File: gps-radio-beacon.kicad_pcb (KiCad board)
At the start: 2 copper layers, 106.4 x 69.7 mm, 40 parts, among them J1 Conn_01x16, J2 Conn_01x16, J3 Conn_Coaxial, J4 Conn_Coaxial, J5 Screw_Terminal_01x04, P1 USB_C_Plug_USB2.0, Q1 Q_PMOS_DGS, U1 PGA2040, U2 RFM95W-915S2, U3 MAX-M10S, U4 NCP1117-3.3_SOT223

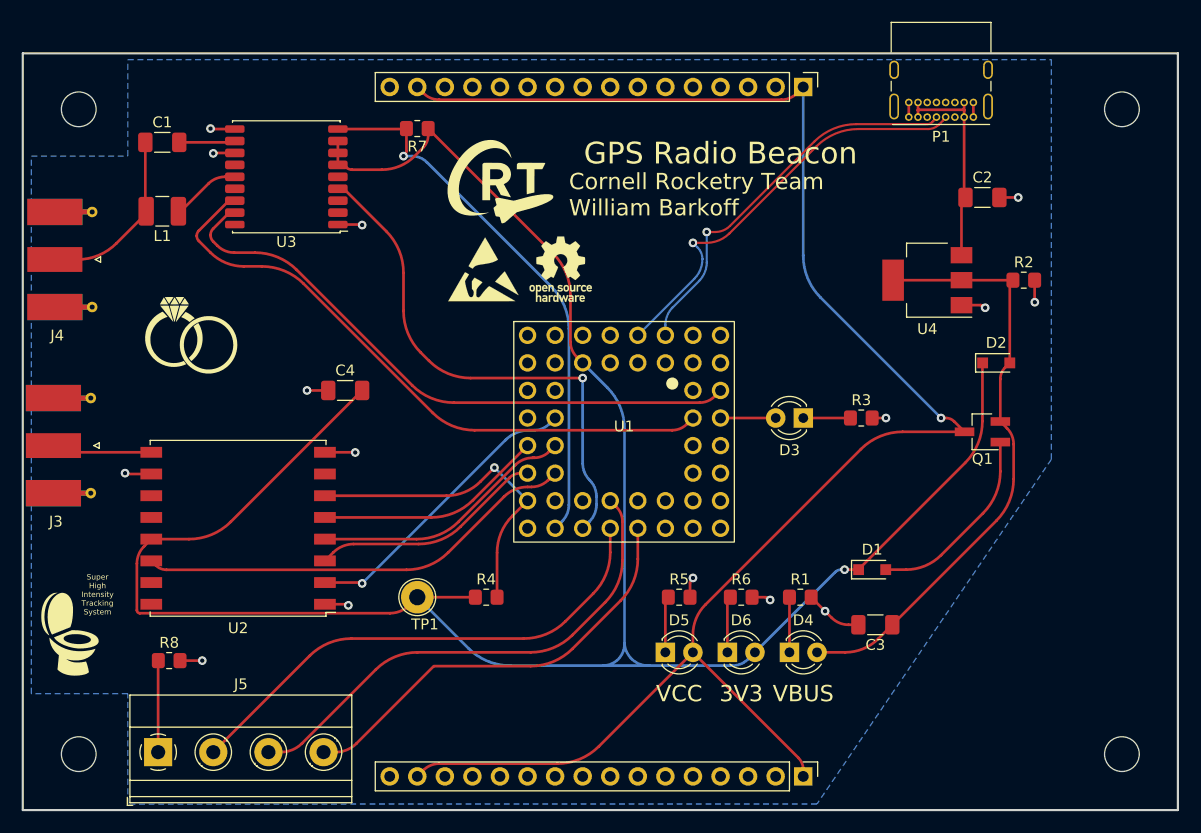
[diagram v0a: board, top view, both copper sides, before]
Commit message: Revert "bendy traces"
This reverts commit 8a4ff923ad6d744258f9f7e3ddda1145dac49418.
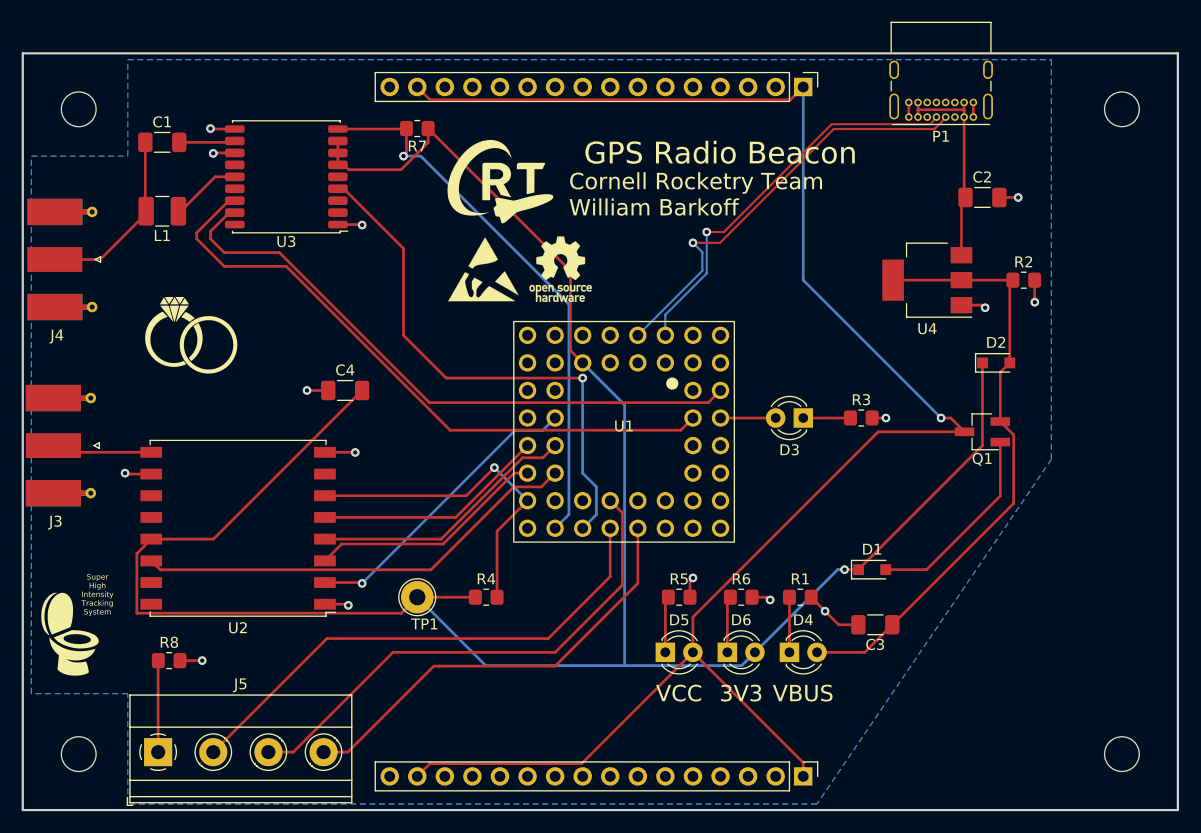
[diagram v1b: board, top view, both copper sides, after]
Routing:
- net VCC: track 154.7 -> 156.1 mm
- net +3V3: track 206.2 -> 205.0 mm
- net /GPS_TIMEPULSE: track 48.2 -> 49.4 mm
- net /IND_LED_2: track 46.2 -> 47.2 mm
- net /GPS_SDA: track 57.9 -> 58.8 mm
- net VBUS: track 55.5 -> 56.4 mm
- net /GPS_SCL: track 56.5 -> 57.3 mm
- net /IND_LED_1: track 46.9 -> 47.7 mm
- net /PWR-USB/USB_D+: track 38.8 -> 39.5 mm
- net /PWR-USB/USB_D-: track 36.1 -> 36.8 mm
- net /IND_LED_3: track 39.8 -> 40.4 mm
- net /RADIO_IRQ: track 40.7 -> 41.2 mm
- net /GPS_RESET: track 50.5 -> 51.0 mm
